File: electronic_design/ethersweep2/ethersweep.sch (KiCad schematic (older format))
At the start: 68 parts, among them J1 AVR-ISP-6, J2 Conn_01x02_Male, J3 Conn_01x04_Female, J4 Conn_01x02_Male, J5 Conn_01x02_Male, J6 HR911105A, J7 Conn_01x06_Female, J8 AVR-ISP-6, J9 Conn_01x06_Male, M1 Stepper_Motor_bipolar, SW1 SW_Push, U1 ENC28J60x-SS, U2 ATmega328-AU, U3 DRV8825PWPR, U4 AMS1117-3.3, U5 AS5600, Y1 Crystal_25MHz, Y3 Crystal

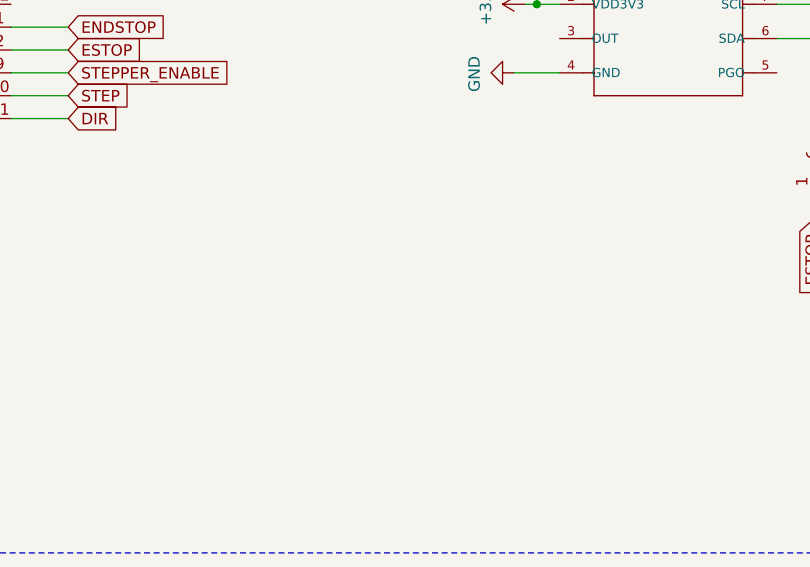
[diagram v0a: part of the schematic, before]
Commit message: cleanup
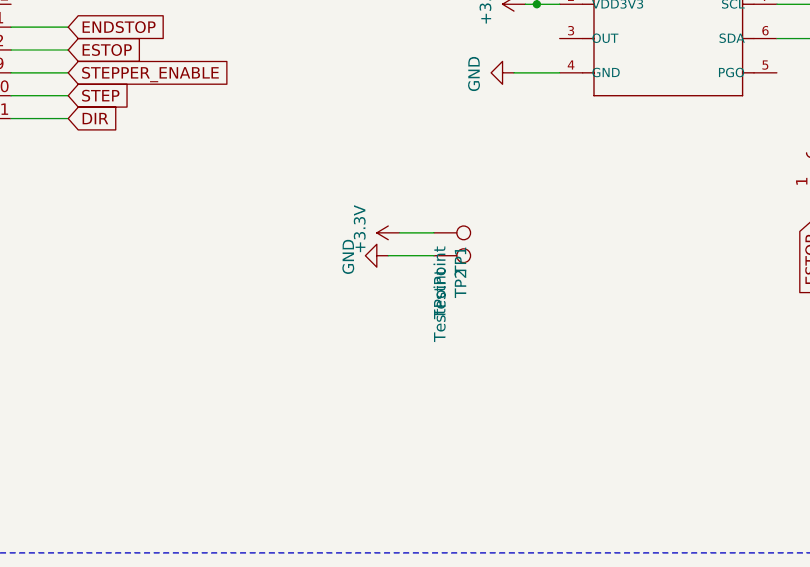
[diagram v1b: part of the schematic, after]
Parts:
- added TP1, TP2: TestPoint, TestPoint:TestPoint_Pad_D2.0mm, symbol Connector:TestPoint
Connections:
- net +3V3: now also TP1.1
- net GND: now also TP2.1
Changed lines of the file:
@@
 	1    0    0    -1
 $EndComp
+$Comp
+L Connector:TestPoint TP1
+U 1 1 603FD0AE
+P 3900 4500
+F 0 "TP1" H 3958 4618 50  0000 L CNN
+F 1 "TestPoint" H 3958 4527 50  0000 L CNN
+F 2 "TestPoint:TestPoint_Pad_D2.0mm" H 4100 4500 50  0001 C CNN
+F 3 "~" H 4100 4500 50  0001 C CNN
+	1    3900 4500
+	0    1    1    0
+$EndComp
+$Comp
+L Connector:TestPoint TP2
+U 1 1 603FE9A9
+P 3900 4600
+F 0 "TP2" H 3958 4718 50  0000 L CNN
+F 1 "TestPoint" H 3958 4627 50  0000 L CNN
+F 2 "TestPoint:TestPoint_Pad_D2.0mm" H 4100 4600 50  0001 C CNN
+F 3 "~" H 4100 4600 50  0001 C CNN
+	1    3900 4600
+	0    1    1    0
+$EndComp
+$Comp
+L power:GND #PWR0143
+U 1 1 6043D76B
+P 3700 4600
+F 0 "#PWR0143" H 3700 4350 50  0001 C CNN
+F 1 "GND" H 3705 4427 50  0000 C CNN
+F 2 "" H 3700 4600 50  0001 C CNN
+F 3 "" H 3700 4600 50  0001 C CNN
+	1    3700 4600
+	0    1    1    0
+$EndComp
+Wire Wire Line
+	3900 4600 3700 4600
+Wire Wire Line
+	3900 4500 3750 4500
+$Comp
+L power:+3.3V #PWR0181
+U 1 1 60452E8B
+P 3750 4500
+F 0 "#PWR0181" H 3750 4350 50  0001 C CNN
+F 1 "+3.3V" H 3765 4673 50  0000 C CNN
+F 2 "" H 3750 4500 50  0001 C CNN
+F 3 "" H 3750 4500 50  0001 C CNN
+	1    3750 4500
+	0    -1   -1   0
+$EndComp
 $EndSCHEMATC
